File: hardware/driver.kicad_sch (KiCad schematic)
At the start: 83 parts, among them J2 BUTTERFLY, J4 SELECTOR, J5 SELECTOR_2, Q1 RJK0355DSP, Q2 RJK0355DSP, Q3 SiRC18DP, Q4 SiRC18DP, Q5 SiRC18DP, Q6 SiRC18DP, U2 LT3743, U3 MAX1978, U4 INA333xxDGK

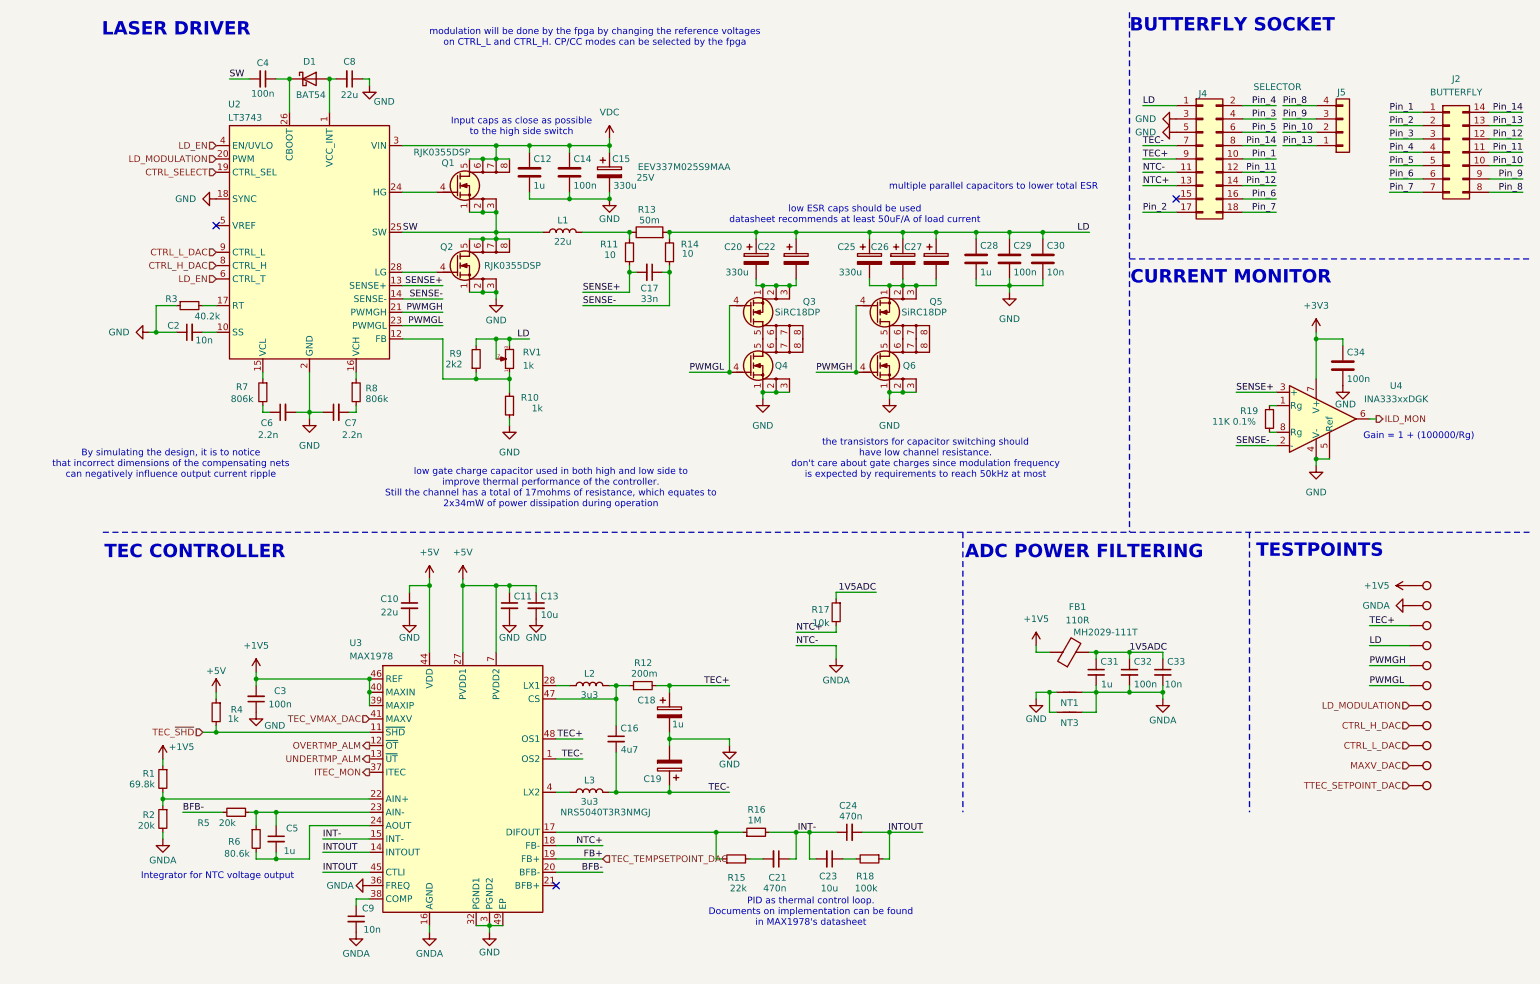
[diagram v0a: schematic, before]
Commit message: fix: tidier schematic
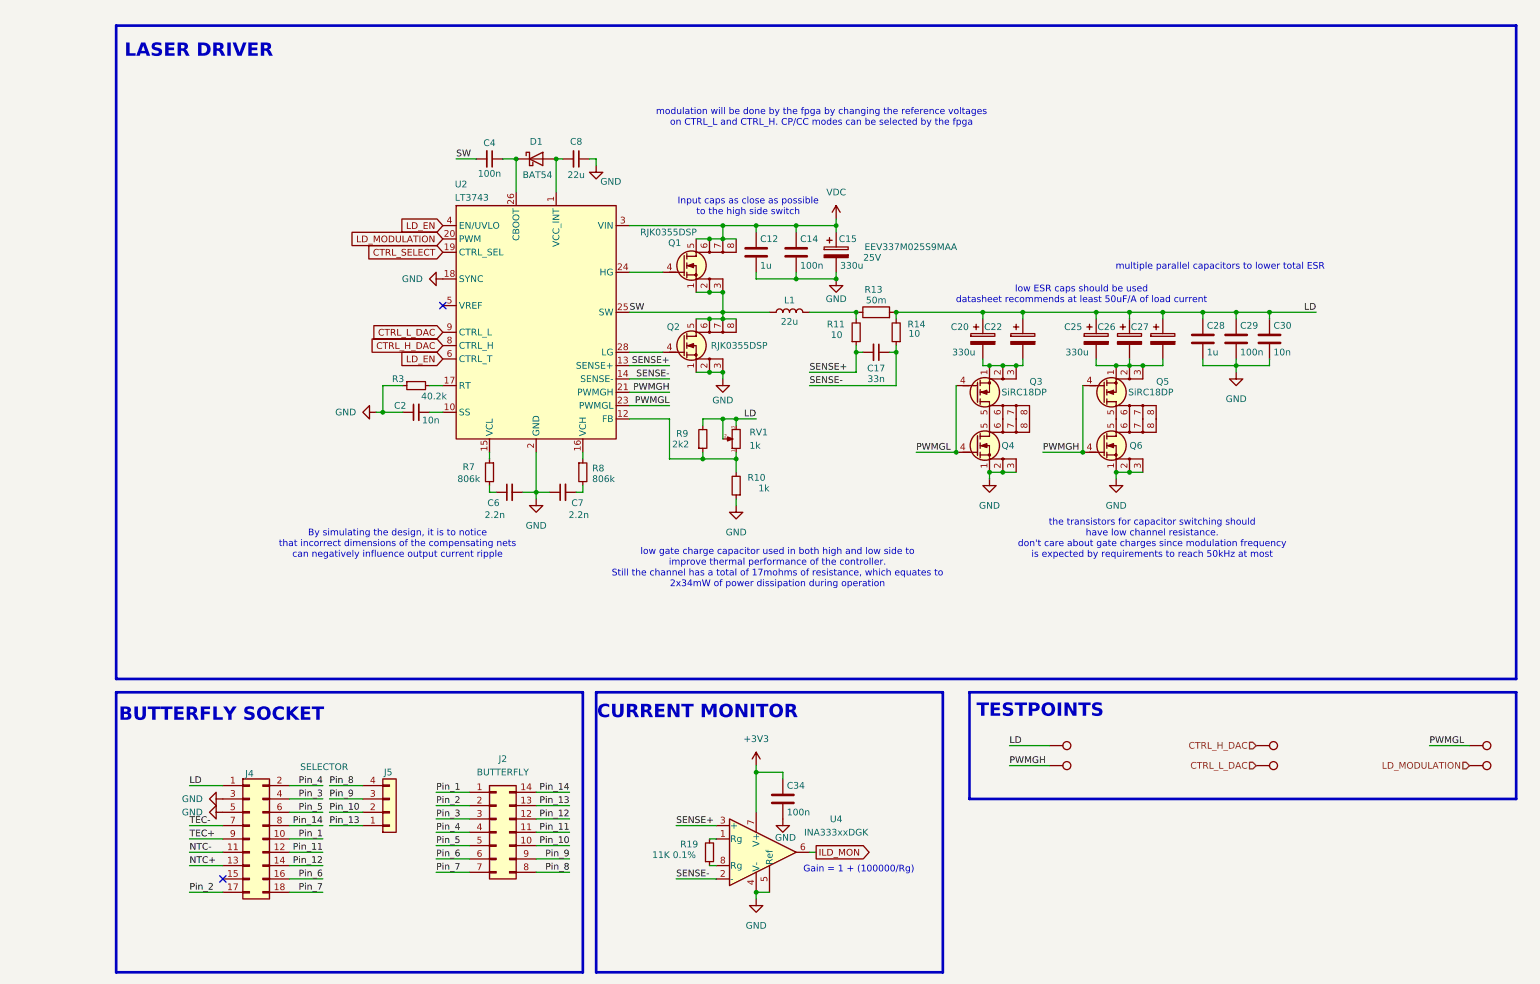
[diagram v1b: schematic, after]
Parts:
- removed C10: 22u, Capacitor_SMD:C_0603_1608Metric, symbol Device:C_Small
- removed C11, C13, C23: 10u, Capacitor_SMD:C_0603_1608Metric, symbol Device:C_Small
- removed C16: 4u7, Capacitor_SMD:C_0603_1608Metric, symbol Device:C_Small
- removed C18, C19: 1u, Capacitor_SMD:CP_Elec_4x5.4, symbol Device:C_Polarized
- removed C21, C24: 470n, Capacitor_SMD:C_0603_1608Metric, symbol Device:C_Small
- removed C3, C32: 100n, Capacitor_SMD:C_0603_1608Metric, symbol Device:C_Small
- removed C31, C5: 1u, Capacitor_SMD:C_0603_1608Metric, symbol Device:C_Small
- removed C33, C9: 10n, Capacitor_SMD:C_0603_1608Metric, symbol Device:C_Small
- removed FB1: 110R, PCM_Ferrite_SMD_AKL:Ferrite_0805_2012Metric, symbol Device:FerriteBead
- removed L2, L3: 3u3, Inductor_SMD:L_Taiyo-Yuden_NR-50xx, symbol Device:L
- removed NT1, NT3: NetTie_2, NetTie:NetTie-2_SMD_Pad0.5mm, symbol Device:NetTie_2
- removed R1: 69.8k, Resistor_SMD:R_0603_1608Metric, symbol Device:R_Small
- removed R12: 200m, PCM_Resistor_SMD_AKL:R_2010_5025Metric, symbol Device:R_Small
- removed R15: 22k, Resistor_SMD:R_0603_1608Metric, symbol Device:R_Small
- removed R16: 1M, Resistor_SMD:R_0603_1608Metric, symbol Device:R_Small
- removed R17: 10k, Resistor_SMD:R_0603_1608Metric, symbol Device:R_Small
- removed R18: 100k, Resistor_SMD:R_0603_1608Metric, symbol Device:R_Small
- removed R2, R5: 20k, Resistor_SMD:R_0603_1608Metric, symbol Device:R_Small
- removed R4: 1k, Resistor_SMD:R_0603_1608Metric, symbol Device:R_Small
- removed R6: 80.6k, Resistor_SMD:R_0603_1608Metric, symbol Device:R_Small
- removed TP1, TP10, TP11: TestPoint, TestPoint:TestPoint_Pad_D1.0mm, symbol Connector:TestPoint
- removed TP2: TestPoint, TestPoint:TestPoint_Pad_1.5x1.5mm, symbol Connector:TestPoint
- removed TP3: TestPoint, TestPoint:TestPoint_Pad_D1.5mm, symbol Connector:TestPoint
- removed U3: MAX1978, Package_DFN_QFN:TQFN-48-1EP_7x7mm_P0.5mm_EP5.1x5.1mm, symbol symbols:MAX1978
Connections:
- net AGND renamed NTC-
- no-connect marks 3 -> 2
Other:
- note removed: "ADC POWER FILTERING"
- note removed: "Integrator for NTC voltage output"
- note removed: "PID as thermal control loop. Documents on implementation can be found in MAX1978's datasheet"
- note removed: "TEC CONTROLLER"
- moved on the sheet: C12, C14, C15, C17, C2, C20, C22, C25, C26, C27, C28, C29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
